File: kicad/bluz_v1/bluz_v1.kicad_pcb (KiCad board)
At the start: 2 copper layers, 24.9 x 14.9 mm, 71 parts, among them J1 USB_B_Micro, J10 Conn, J11 Conn, J12 BTAnt, J2 Conn, J3 Conn, J4 Conn, J5 Conn, J6 Conn, J7 Conn, J8 Conn, J9 Conn, M1 VibroMotor, Q1 RUM002N05, Q2 RUM002N05, SW1 SW_DPDT_x2, U1 MCP73831, U2 MCP1700, U3 TLV3201AIDCK, U4 AP3015KTR, Y1 NX1612SA-32MHz, Y2 NX1610-32.768

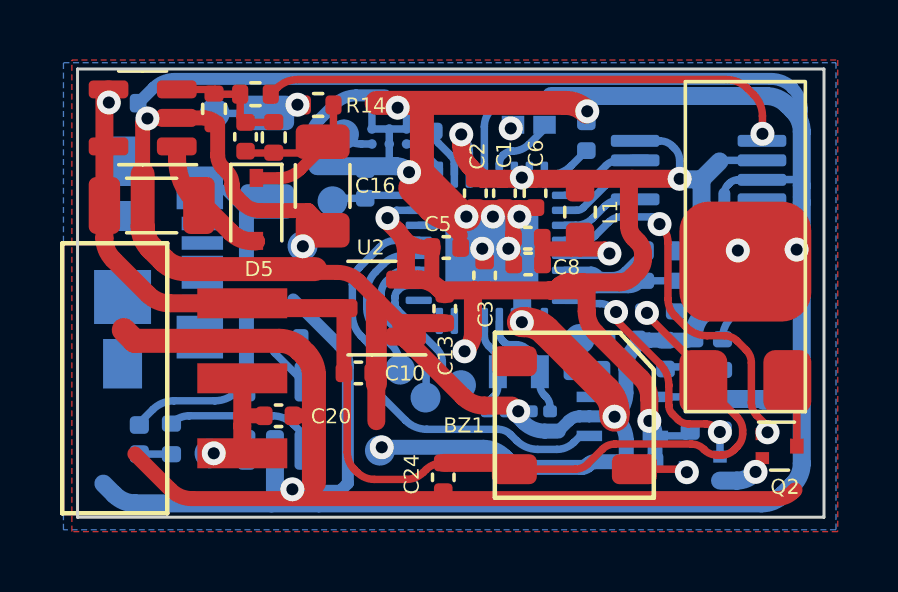
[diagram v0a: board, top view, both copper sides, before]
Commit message: изменено:      kicad/bluz_v1/bluz_v1.kicad_pcb 	изменено:      kicad/bluz_v1/bluz_v1.kicad_sch 	изменено:      stm32cubeide/BluZ_v1/Core/Src/main.c 	изменено:      stm32cubeide/BluZ_v1/Release/Core/Src/subdir.mk 	изменено:      stm32cubeide/BluZ_v1/Release/System/Config/LowPower/peripheral_init.cyclo 	изменено:      stm32cubeide/BluZ_v1/Release/System/Config/LowPower/peripheral_init.su 	изменено:      stm32cubeide/BluZ_v1/Release/System/Interfaces/stm32_lpm_if.cyclo 	изменено:      stm32cubeide/BluZ_v1/Release/System/Interfaces/stm32_lpm_if.su 	изменено:      stm32cubeide/BluZ_v1/Release/System/Interfaces/timer_if.cyclo 	изменено:      stm32cubeide/BluZ_v1/Release/System/Interfaces/timer_if.su 	изменено:      stm32cubeide/BluZ_v1/Release/System/Interfaces/usart_if.cyclo 	изменено:      stm32cubeide/BluZ_v1/Release/System/Interfaces/usart_if.su 	изменено:      stm32cubeide/BluZ_v1/Release/System/Modules/scm.cyclo 	изменено:      stm32cubeide/BluZ_v1/Release/System/Modules/scm.su 	изменено:      stm32cubeide/BluZ_v1/Release/objects.list
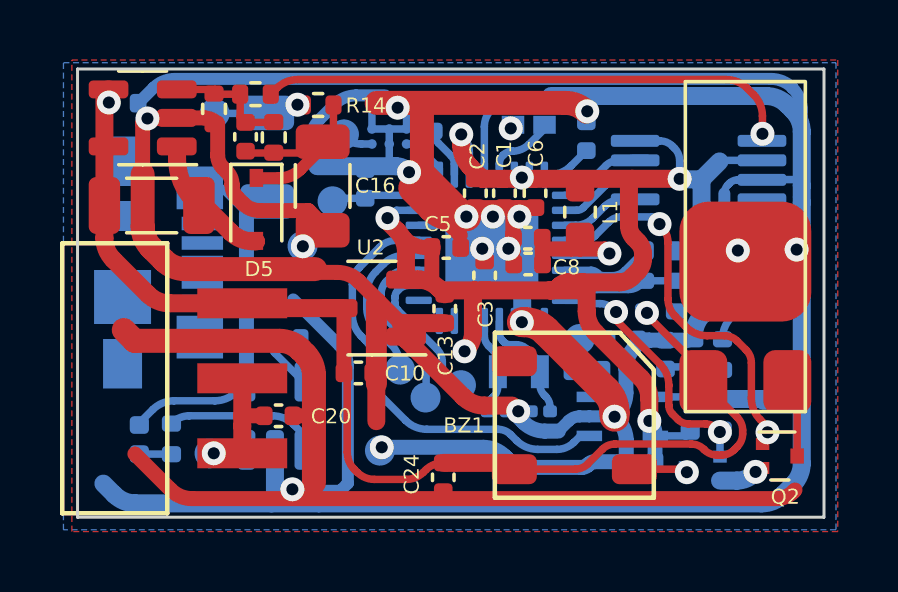
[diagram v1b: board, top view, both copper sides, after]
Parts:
- moved Q2 0.33 mm to (85.1, 50.0)
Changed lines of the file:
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@@
   )
   (footprint "My-library:SOT-723" (layer "F.Cu")
-    (at 85.1 49.68)
+    (at 85.11 50.01)
     (descr "http://toshiba.semicon-storage.com/info/docget.jsp?did=5879&prodName=RN1104MFV")
     (tags "sot 723")
@@
   (segment (start 78.44 46.11) (end 78.276714 46.11) (width 0.25) (layer "B.Cu") (net 11))
   (arc (start 77.569607 45.817107) (mid 77.89403 46.03388) (end 78.276714 46.11) (width 0.25) (layer "B.Cu") (net 11))
+  (segment (start 83.685736 46.175736) (end 83.984264 46.474264) (width 0.25) (layer "F.Cu") (net 12))
+  (segment (start 81.614314 45.344314) (end 81.977107 45.707107) (width 0.25) (layer "F.Cu") (net 12))
   (segment (start 81.1 42.28) (end 81.145685 42.325685) (width 0.25) (layer "F.Cu") (net 12))
-  (segment (start 84.16 46.898528) (end 84.16 48.231472) (width 0.25) (layer "F.Cu") (net 12))
-  (segment (start 81.614314 45.344314) (end 81.977107 45.707107) (width 0.25) (layer "F.Cu") (net 12))
-  (segment (start 84.7 49.02) (end 84.7 49.22) (width 0.25) (layer "F.Cu") (net 12))
-  (segment (start 84.335736 48.655736) (end 84.7 49.02) (width 0.25) (layer "F.Cu") (net 12))
+  (segment (start 84.535 49.61) (end 84.535 49.385) (width 0.25) (layer "F.Cu") (net 12))
+  (segment (start 84.452893 48.792893) (end 84.7 49.04) (width 0.25) (layer "F.Cu") (net 12))
+  (segment (start 82.684214 46) (end 83.261472 46) (width 0.25) (layer "F.Cu") (net 12))
+  (segment (start 84.535 49.385) (end 84.7 49.22) (width 0.25) (layer "F.Cu") (net 12))
+  (segment (start 84.16 46.898528) (end 84.16 48.085786) (width 0.25) (layer "F.Cu") (net 12))
+  (segment (start 84.7 49.04) (end 84.7 49.22) (width 0.25) (layer "F.Cu") (net 12))
   (segment (start 81.38 42.891371) (end 81.38 44.778629) (width 0.25) (layer "F.Cu") (net 12))
-  (segment (start 83.685736 46.175736) (end 83.984264 46.474264) (width 0.25) (layer "F.Cu") (net 12))
-  (segment (start 82.684214 46) (end 83.261472 46) (width 0.25) (layer "F.Cu") (net 12))
   (via (at 84.7 49.22) (size 0.8) (drill 0.4) (layers "F.Cu" "B.Cu") (net 12))
   (via (at 81.1 42.28) (size 0.8) (drill 0.4) (layers "F.Cu" "B.Cu") (free) (net 12))
-  (arc (start 84.335736 48.655736) (mid 84.205672 48.461082) (end 84.16 48.231472) (width 0.25) (layer "F.Cu") (net 12))
+  (arc (start 83.261472 46) (mid 83.491082 46.045672) (end 83.685736 46.175736) (width 0.25) (layer "F.Cu") (net 12))
+  (arc (start 84.452893 48.792893) (mid 84.23612 48.46847) (end 84.16 48.085786) (width 0.25) (layer "F.Cu") (net 12))
   (arc (start 81.145685 42.325685) (mid 81.319103 42.585224) (end 81.38 42.891371) (width 0.25) (layer "F.Cu") (net 12))
   (arc (start 81.38 44.778629) (mid 81.440896 45.084775) (end 81.614314 45.344314) (width 0.25) (layer "F.Cu") (net 12))
   (arc (start 83.984264 46.474264) (mid 84.114328 46.668918) (end 84.16 46.898528) (width 0.25) (layer "F.Cu") (net 12))
-  (arc (start 83.261472 46) (mid 83.491082 46.045672) (end 83.685736 46.175736) (width 0.25) (layer "F.Cu") (net 12))
   (arc (start 81.977107 45.707107) (mid 82.301531 45.92388) (end 82.684214 46) (width 0.25) (layer "F.Cu") (net 12))
   (segment (start 77.9475 42.82) (end 78.592893 42.82) (width 0.25) (layer "B.Cu") (net 12))
@@
   (arc (start 78.697157 44.32) (mid 78.773694 44.335224) (end 78.838579 44.378579) (width 0.25) (layer "B.Cu") (net 37))
   (arc (start 80.485736 44.284264) (mid 80.291082 44.414328) (end 80.061472 44.46) (width 0.25) (layer "B.Cu") (net 37))
-  (segment (start 85.675 47.845) (end 85.36 47.53) (width 0.25) (layer "F.Cu") (net 38))
-  (segment (start 85.675 49.68) (end 85.675 47.845) (width 0.25) (layer "F.Cu") (net 38))
+  (segment (start 85.685 47.855) (end 85.36 47.53) (width 0.25) (layer "F.Cu") (net 38))
+  (segment (start 85.685 50.01) (end 85.685 47.855) (width 0.25) (layer "F.Cu") (net 38))
   (segment (start 65.603287 41.518287) (end 65.745 41.66) (width 0.6) (layer "F.Cu") (net 39))
   (segment (start 65.0175 39.75) (end 65.0175 40.104073) (width 0.6) (layer "F.Cu") (net 39))
